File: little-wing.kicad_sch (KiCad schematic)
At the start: 72 parts, among them IC1 AP7335-WG-7, J1 nice!view, J2 Battery, J3 trackball, J4 trackball, SW1 Power, SW2 Reset, U1 nice!nano v2, U2 PMW3610

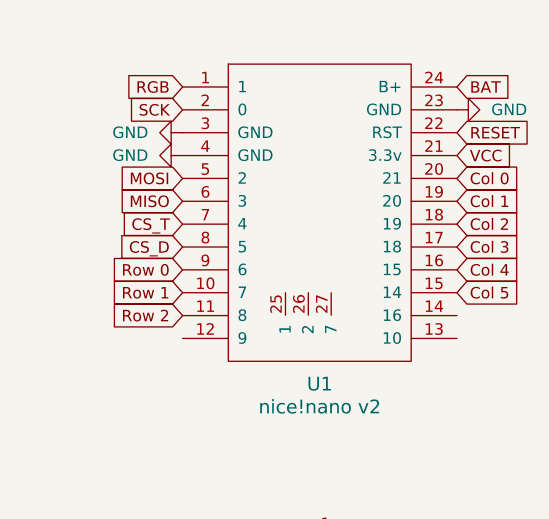
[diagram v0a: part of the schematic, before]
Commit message: Wiring up the MCU block
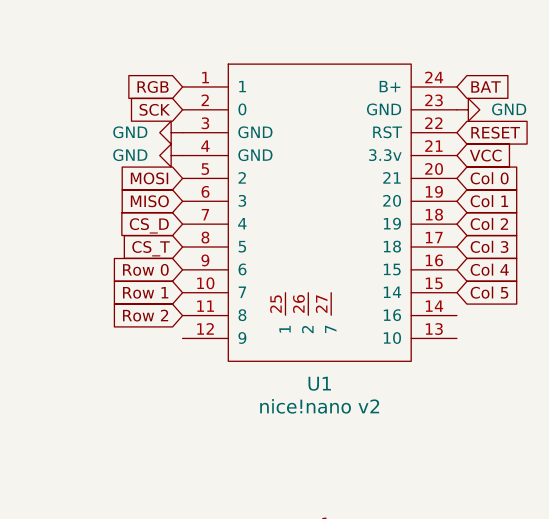
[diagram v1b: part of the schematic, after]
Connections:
- net CS_D: now also U1.7 (4); no longer U1.8 (5)
- net CS_T: now also U1.8 (5); no longer U1.7 (4)
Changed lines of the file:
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@@
+		)
+	)
+	(global_label "CS_T"
+		(shape input)
+		(at 35.56 41.91 180)
+		(fields_autoplaced yes)
+		(effects
+			(font
+				(size 1.27 1.27)
+			)
+			(justify right)
+		)
+		(property "Intersheetrefs" "${INTERSHEET_REFS}"
+			(at 28.1601 41.91 0)
+			(effects
+				(font
+					(size 1.27 1.27)
+				)
+				(justify right)
+				(hide yes)
+			)
 		)
 	)
@@
 		)
 	)
+	(global_label "CS_D"
+		(shape input)
+		(at 35.56 39.37 180)
+		(fields_autoplaced yes)
+		(effects
+			(font
+				(size 1.27 1.27)
+			)
+			(justify right)
+		)
+		(property "Intersheetrefs" "${INTERSHEET_REFS}"
+			(at 27.8577 39.37 0)
+			(effects
+				(font
+					(size 1.27 1.27)
+				)
+				(justify right)
+				(hide yes)
+			)
+		)
+	)
 	(global_label "GND"
 		(shape input)
@@
 		)
 	)
-	(global_label "CS_D"
-		(shape input)
-		(at 35.56 41.91 180)
-		(fields_autoplaced yes)
-		(effects
-			(font
-				(size 1.27 1.27)
-			)
-			(justify right)
-		)
-		(property "Intersheetrefs" "${INTERSHEET_REFS}"
-			(at 27.8577 41.91 0)
-			(effects
-				(font
-					(size 1.27 1.27)
-				)
-				(justify right)
-				(hide yes)
-			)
-		)
-	)
 	(global_label "Row 0"
 		(shape input)
@@
 			(effects
 				(font
-					(size 1.27 1.27)
-				)
-				(justify right)
-				(hide yes)
-			)
-		)
-	)
-	(global_label "CS_T"
-		(shape input)
-		(at 35.56 39.37 180)
-		(fields_autoplaced yes)
-		(effects
-			(font
-				(size 1.27 1.27)
-			)
-			(justify right)
-		)
-		(property "Intersheetrefs" "${INTERSHEET_REFS}"
-			(at 28.1601 39.37 0)
-			(effects
-				(font
